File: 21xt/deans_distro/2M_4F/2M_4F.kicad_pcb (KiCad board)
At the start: 6 copper layers, 31.2 x 36.5 mm, 6 parts, among them J1 Conn_01x02, J2 Conn_01x02, J3 Conn_01x02, J4 Conn_01x02, J5 Conn_01x02, J6 Conn_01x02

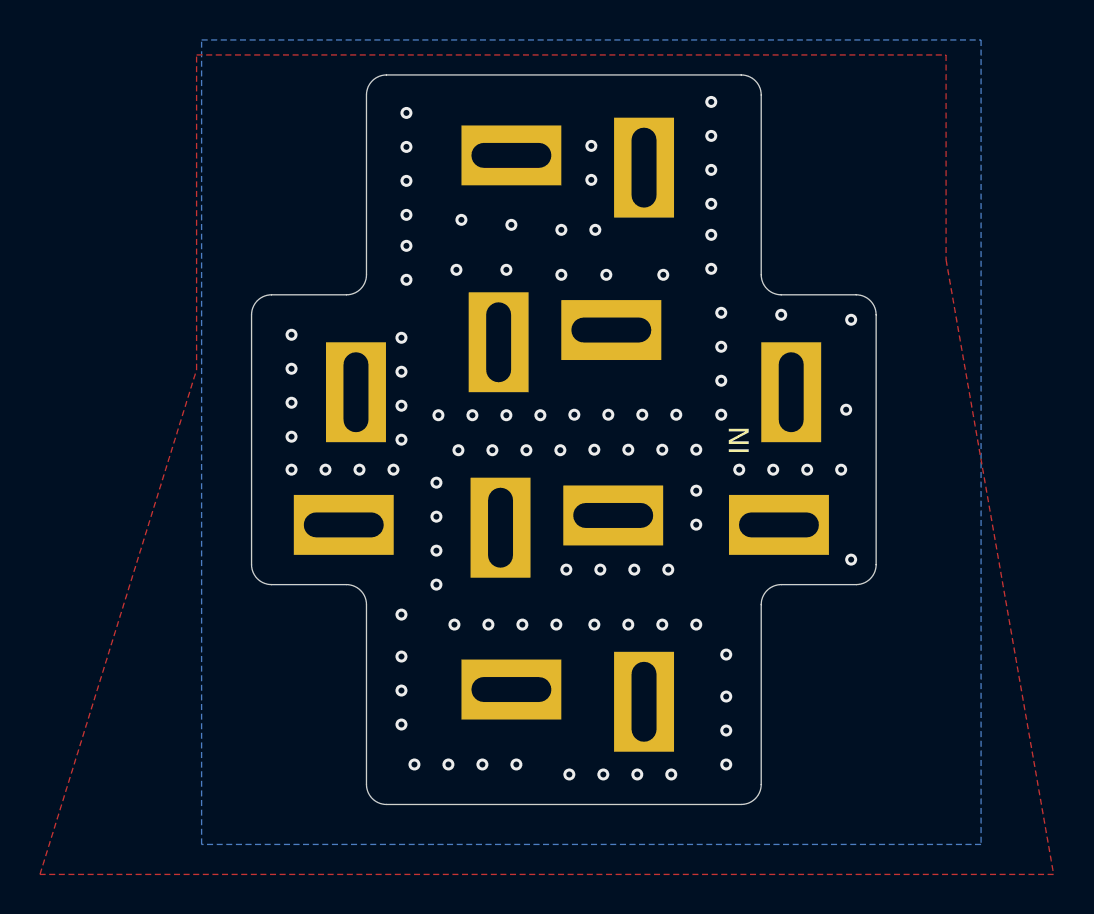
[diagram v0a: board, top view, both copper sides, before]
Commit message: adf
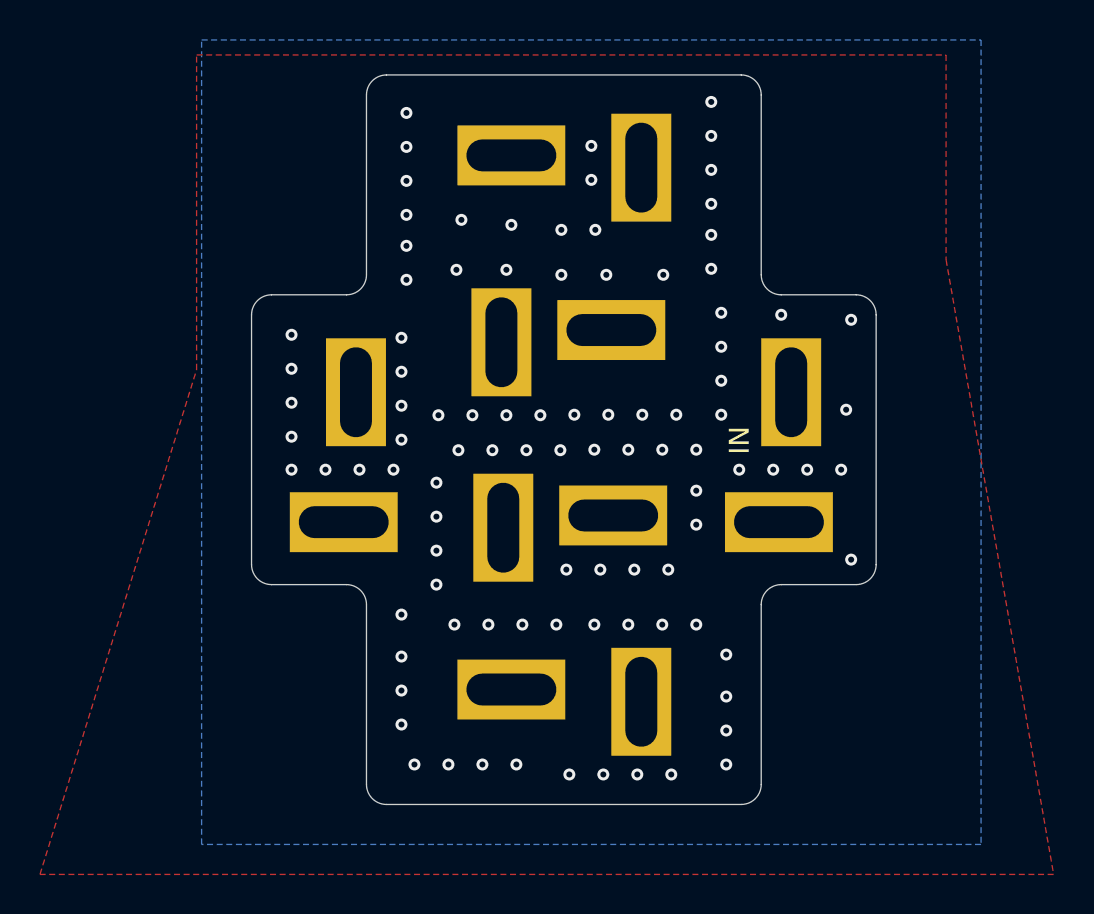
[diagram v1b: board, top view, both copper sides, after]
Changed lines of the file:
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@@
 		)
 		(pad "1" thru_hole rect
-			(at 4.25 3.3625 270)
-			(size 5 3)
-			(drill oval 4 1.25)
+			(at 4.25 3.5 270)
+			(size 5.4 3)
+			(drill oval 4.5 1.6)
 			(layers "*.Cu" "*.Mask")
 			(remove_unused_layers no)
@@
 		(pad "2" thru_hole rect
 			(at 4.8625 9)
-			(size 5 3)
-			(drill oval 4 1.25)
+			(size 5.4 3)
+			(drill oval 4.5 1.6)
 			(layers "*.Cu" "*.Mask")
 			(remove_unused_layers no)
@@
 		)
 		(pad "1" thru_hole rect
-			(at 4.25 3.3625 270)
-			(size 5 3)
-			(drill oval 4 1.25)
+			(at 4.25 3.5 270)
+			(size 5.4 3)
+			(drill oval 4.5 1.6)
 			(layers "*.Cu" "*.Mask")
 			(remove_unused_layers no)
@@
 		(pad "2" thru_hole rect
 			(at 4.8625 9)
-			(size 5 3)
-			(drill oval 4 1.25)
+			(size 5.4 3)
+			(drill oval 4.5 1.6)
 			(layers "*.Cu" "*.Mask")
 			(remove_unused_layers no)
@@
 		)
 		(pad "1" thru_hole rect
-			(at 4.25 -2.3625 90)
-			(size 5 3)
-			(drill oval 4 1.25)
+			(at 4.25 -2.5 90)
+			(size 5.4 3)
+			(drill oval 4.5 1.6)
 			(layers "*.Cu" "*.Mask")
 			(remove_unused_layers no)
@@
 		(pad "2" thru_hole rect
 			(at 4.8625 -9)
-			(size 5 3)
-			(drill oval 4 1.25)
+			(size 5.4 3)
+			(drill oval 4.5 1.6)
 			(layers "*.Cu" "*.Mask")
 			(remove_unused_layers no)
@@
 		(model "C:/Users/justin/Documents/bjr_kicad/21xt/deans_distro/deans_3dmodel/T-Plug female - W.S Deans Co. Est. 1957.step"
 			(offset
-				(xyz 4.35 -6.35 10.5)
+				(xyz 4.35 -6.55 10.5)
 			)
 			(scale
@@
 		)
 		(pad "1" thru_hole rect
-			(at 4.25 -2.3625)
-			(size 5 3)
-			(drill oval 4 1.25)
+			(at 4.25 -2.5)
+			(size 5.4 3)
+			(drill oval 4.5 1.6)
 			(layers "*.Cu" "*.Mask")
 			(remove_unused_layers no)
@@
 		(pad "2" thru_hole rect
 			(at 4.8625 -9 270)
-			(size 5 3)
-			(drill oval 4 1.25)
+			(size 5.4 3)
+			(drill oval 4.5 1.6)
 			(layers "*.Cu" "*.Mask")
 			(remove_unused_layers no)
@@
 		(model "C:/Users/justin/Documents/bjr_kicad/21xt/deans_distro/deans_3dmodel/T-Plug female - W.S Deans Co. Est. 1957.step"
 			(offset
-				(xyz 4.35 -6.35 10.5)
+				(xyz 4.35 -6.55 10.5)
 			)
 			(scale
@@
 		)
 		(pad "1" thru_hole rect
-			(at 4.25 -2.3625 90)
-			(size 5 3)
-			(drill oval 4 1.25)
+			(at 4.25 -2.5 90)
+			(size 5.4 3)
+			(drill oval 4.5 1.6)
 			(layers "*.Cu" "*.Mask")
 			(remove_unused_layers no)
@@
 		(pad "2" thru_hole rect
 			(at 4.8625 -9)
-			(size 5 3)
-			(drill oval 4 1.25)
+			(size 5.4 3)
+			(drill oval 4.5 1.6)
 			(layers "*.Cu" "*.Mask")
 			(remove_unused_layers no)
@@
 		(model "C:/Users/justin/Documents/bjr_kicad/21xt/deans_distro/deans_3dmodel/T-Plug female - W.S Deans Co. Est. 1957.step"
 			(offset
-				(xyz 4.35 -6.35 10.5)
+				(xyz 4.35 -6.55 10.5)
 			)
 			(scale
@@
 		)
 		(pad "1" thru_hole rect
-			(at 4.25 -2.3625)
-			(size 5 3)
-			(drill oval 4 1.25)
+			(at 4.25 -2.5)
+			(size 5.4 3)
+			(drill oval 4.5 1.6)
 			(layers "*.Cu" "*.Mask")
 			(remove_unused_layers no)
@@
 		(pad "2" thru_hole rect
 			(at 4.8625 -9 270)
-			(size 5 3)
-			(drill oval 4 1.25)
+			(size 5.4 3)
+			(drill oval 4.5 1.6)
 			(layers "*.Cu" "*.Mask")
 			(remove_unused_layers no)
@@
 		(model "C:/Users/justin/Documents/bjr_kicad/21xt/deans_distro/deans_3dmodel/T-Plug female - W.S Deans Co. Est. 1957.step"
 			(offset
-				(xyz 4.35 -6.35 10.5)
+				(xyz 4.35 -6.55 10.5)
 			)
 			(scale
